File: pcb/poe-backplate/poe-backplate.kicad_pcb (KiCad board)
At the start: 6 copper layers, 59.2 x 75 mm, 113 parts, among them IC1 LAN9500A-ABZJ, IC2 93LC66AT-I_OT, J3 USB_C_Receptacle_USB2.0_14P, J4 USB_C_Receptacle_USB2.0_14P, J5 Conn_02x04_Counter_Clockwise, U1 LP38693MP-3.3, U2 HY931147C, U5 USBLC6-2SC6, Y1 ECS-250-18-36B2-CTY-TR

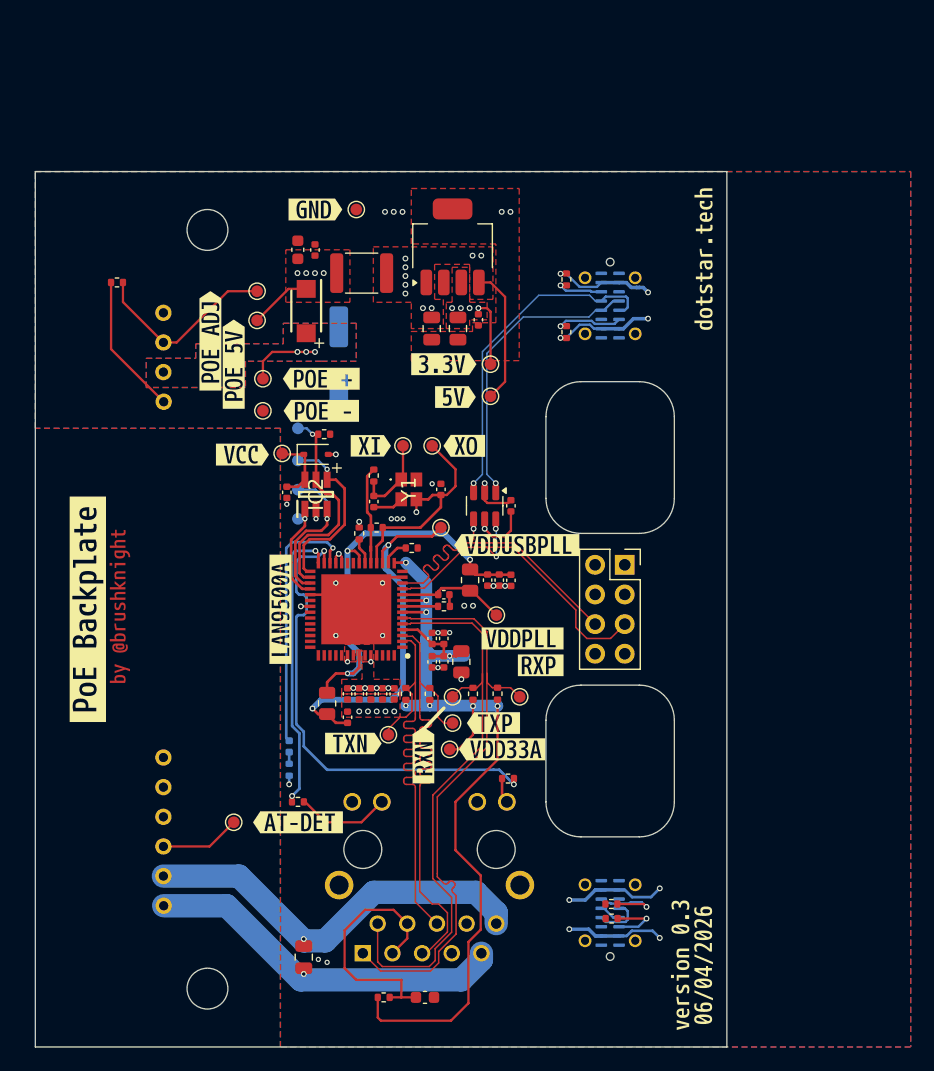
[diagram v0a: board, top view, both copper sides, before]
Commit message: PoE backplate
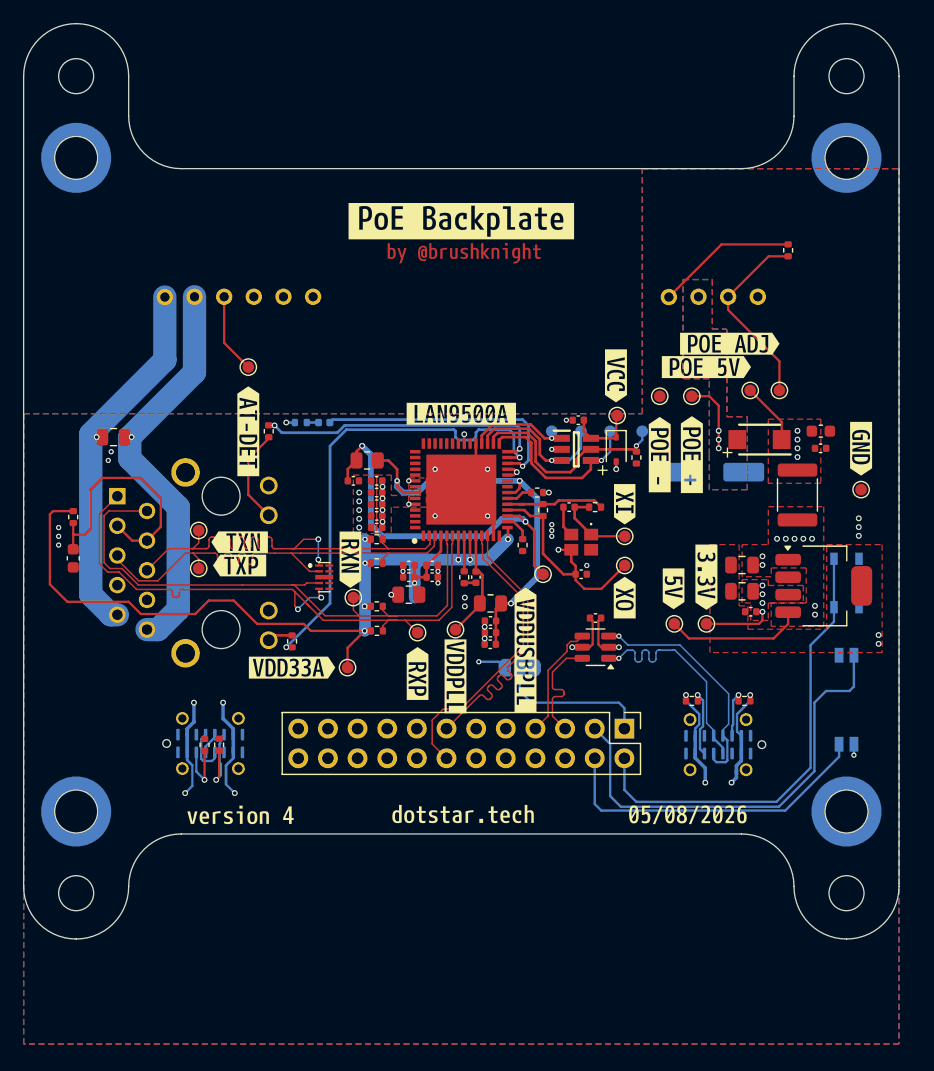
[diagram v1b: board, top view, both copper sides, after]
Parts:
- removed kibuzzard-697BD4F1: G***, kibuzzard-697BD4F1
- removed kibuzzard-697F855F: G***, kibuzzard-697F855F
- removed kibuzzard-697F8566: G***, kibuzzard-697F8566
- removed kibuzzard-697F858D: G***, kibuzzard-697F858D
- removed kibuzzard-69D3A526: G***, kibuzzard-69D3A526
- removed kibuzzard-69D3A52E: G***, kibuzzard-69D3A52E
- added D4: RCLAMP0524PATCT, RCLAMP0524PATCT:RCLAMP0524PATCT, F.Cu at (65.8, 75.8)
- added H1: MountingHole_Pad, 9774030151R:9774030151R, B.Cu at (44.5, 39.8)
- added H2: MountingHole_Pad, 9774030151R:9774030151R, B.Cu at (110.5, 39.8)
- added H3: MountingHole_Pad, 9774030151R:9774030151R, B.Cu at (110.5, 95.8)
- added H4: MountingHole_Pad, 9774030151R:9774030151R, B.Cu at (44.5, 95.8)
- added JP1: SolderJumper_3_Open, Jumper:SolderJumper-3_P1.3mm_Open_RoundedPad1.0x1.5mm_NumberLabels, B.Cu at (82.5, 83.5)
- added S6: 218-2LPSTRF, 218-2LPSTRF:2182LPSTRF, B.Cu at (110.5, 86.2)
- added SW1: power reset, Button_Switch_SMD:SW_SPST_PTS810, B.Cu at (110.5, 76.2)
- added kibuzzard-6A266BA6: G***, kibuzzard-6A266BA6, B.Cu at (105.3, 83.1)
- added kibuzzard-6A266BBE: G***, kibuzzard-6A266BBE, B.Cu at (106.5, 76.0)
- added kibuzzard-6A416FC5: G***, kibuzzard-6A416FC5, B.Cu at (99.5, 96.0)
- added kibuzzard-6A416FFB: G***, kibuzzard-6A416FFB, B.Cu at (56.3, 95.9)
- added kibuzzard-6A58C3F0: G***, kibuzzard-6A58C3F0, F.Cu at (77.0, 84.2)
- added kibuzzard-6A58C460: G***, kibuzzard-6A58C460, F.Cu at (58.5, 72.8)
- added kibuzzard-6A58C49B: G***, kibuzzard-6A58C49B, F.Cu at (73.8, 84.0)
- added kibuzzard-6A58C4AC: G***, kibuzzard-6A58C4AC, F.Cu at (63.0, 83.5)
- added kibuzzard-6A7327CD: G***, kibuzzard-6A7327CD, F.Cu at (58.6, 96.1)
- added kibuzzard-6A7327D6: G***, kibuzzard-6A7327D6, F.Cu at (96.9, 96.1)
- J5: value Conn_02x04_Counter_Clockwise -> Conn_02x12_Counter_Clockwise; footprint Connector_PinSocket_2.54mm:PinSocket_2x04_P2.54mm_Vertical -> Connector_PinHeader_2.54mm:PinHeader_2x12_P2.54mm_Vertical
- moved R19 57.6 mm to (105.5, 47.8), turned to 90 degrees
- moved kibuzzard-6985C4FD 51.8 mm to (77.6, 96.0), turned to 0 degrees
- moved kibuzzard-6978AB9F 51.0 mm to (111.8, 64.8), turned to -90 degrees
- moved TP1 49.5 mm to (111.8, 68.2), turned to -90 degrees
- moved R14 49.0 mm to (44.2, 70.6), turned to -90 degrees
- moved C23 48.2 mm to (44.2, 74.1), turned to -90 degrees
- moved C24 47.4 mm to (47.7, 63.8), turned to 0 degrees
- moved C21 47.4 mm to (108.3, 63.2), turned to 0 degrees
- moved C22 46.5 mm to (108.3, 64.7), turned to 0 degrees
- moved kibuzzard-6985C516 46.1 mm to (77.5, 45.2), turned to 0 degrees
- moved TP7 45.6 mm to (104.8, 59.8), turned to -90 degrees
- moved kibuzzard-68DA54A3 44.5 mm to (100.5, 55.8), turned to 0 degrees
- moved POE1 43.3 mm to (62.3, 51.7), turned to -90 degrees
- moved U1 43.1 mm to (108.5, 76.5), turned to 0 degrees
- moved TP10 42.7 mm to (102.2, 59.8), turned to -90 degrees
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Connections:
- net Net-(POE1-VIN+) renamed /PoE/POE_VIN+
- net Net-(POE1-VIN-) renamed /PoE/POE_VIN-
- J5 pad 1: unconnected-(J5-Pin_1-Pad1) -> /USB to Ethernet/USB_OTG_SWITCH
- J5 pad 2: unconnected-(J5-Pin_2-Pad2) -> /USB to Ethernet/GLOBAL_EN
- J5 pad 3: unconnected-(J5-Pin_3-Pad3) -> /USB to Ethernet/OTG_MODE_SW1
- J5 pad 4: unconnected-(J5-Pin_4-Pad4) -> /USB to Ethernet/nRPIBOOT
- J5 pad 5: /USB to Ethernet/USBDN -> /USB to Ethernet/USBD_POGO_N
- J5 pad 6: /USB to Ethernet/USBDP -> /USB to Ethernet/EEPROM_nWP
- J5 pad 7: +5V -> /USB to Ethernet/USBD_POGO_P
- J5 pad 8: GND -> unconnected-(J5-Pin_8-Pad8)
- U5 pad 4: /USB to Ethernet/USBDP -> /USB to Ethernet/USBD_POGO_P
- U5 pad 6: /USB to Ethernet/USBDN -> /USB to Ethernet/USBD_POGO_N
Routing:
- net /USB to Ethernet/GLOBAL_EN: track 0.00 -> 39.0 mm
- net /USB to Ethernet/OTG_MODE_SW1: track 0.00 -> 38.0 mm
- net /USB to Ethernet/nRPIBOOT: track 0.00 -> 28.1 mm
- net /USB to Ethernet/USB_OTG_SWITCH: track 0.00 -> 13.3 mm
- net /USB to Ethernet/USBD_POGO_P: track 0.00 -> 9.90 mm
- net /USB to Ethernet/USBD_POGO_N: track 0.00 -> 9.87 mm
- net /PoE/POE_5V: track 121.6 -> 112.9 mm
- net /USB to Ethernet/USB_D+: track 28.1 -> 20.2 mm
- net /USB to Ethernet/USB_D-: track 24.6 -> 19.6 mm
- net /USB to Ethernet/USBDN: track 29.1 -> 25.4 mm, vias 2 -> 0
- net /PoE/TXP: track 43.8 -> 40.4 mm
- net /PoE/RXP: track 51.5 -> 54.7 mm, vias 0 -> 2
- net +3.3V: track 10.2 -> 12.6 mm, vias 16 -> 17
- net /PoE/VDD33A: track 83.9 -> 81.8 mm
- net /USB to Ethernet/USBDP: track 26.8 -> 25.0 mm, vias 1 -> 0
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- added copper zone on In3.Cu, net +3.3V
- added copper zone on In1.Cu, net GND
- removed copper zone on In1.Cu, net +3.3V
- removed copper zone on In3.Cu, net GND
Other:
- board size 59.2 x 75 mm -> 75 x 78.4 mm
